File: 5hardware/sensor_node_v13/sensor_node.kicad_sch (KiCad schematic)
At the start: 42 parts, among them J1 Conn_01x08_Socket, J2 Conn_01x08_Socket, Q1 AO3400A, Q2 AO3401A, Q4 AO3401A, SW1 SW_Push, SW2 SW_Push, SW3 SW_Push, SW4 SW_Reed, SW5 SW_Push, SW6 SW_Push, SW7 SW_Push, U1 ESP-12F, U12 APDS-9960, U13 SHT31-DIS, U17 BH1750FVI-TR, U2 2N7002DW, U3 INA219AxDCN, U7 XC6206PxxxMR, U8 TPL5110

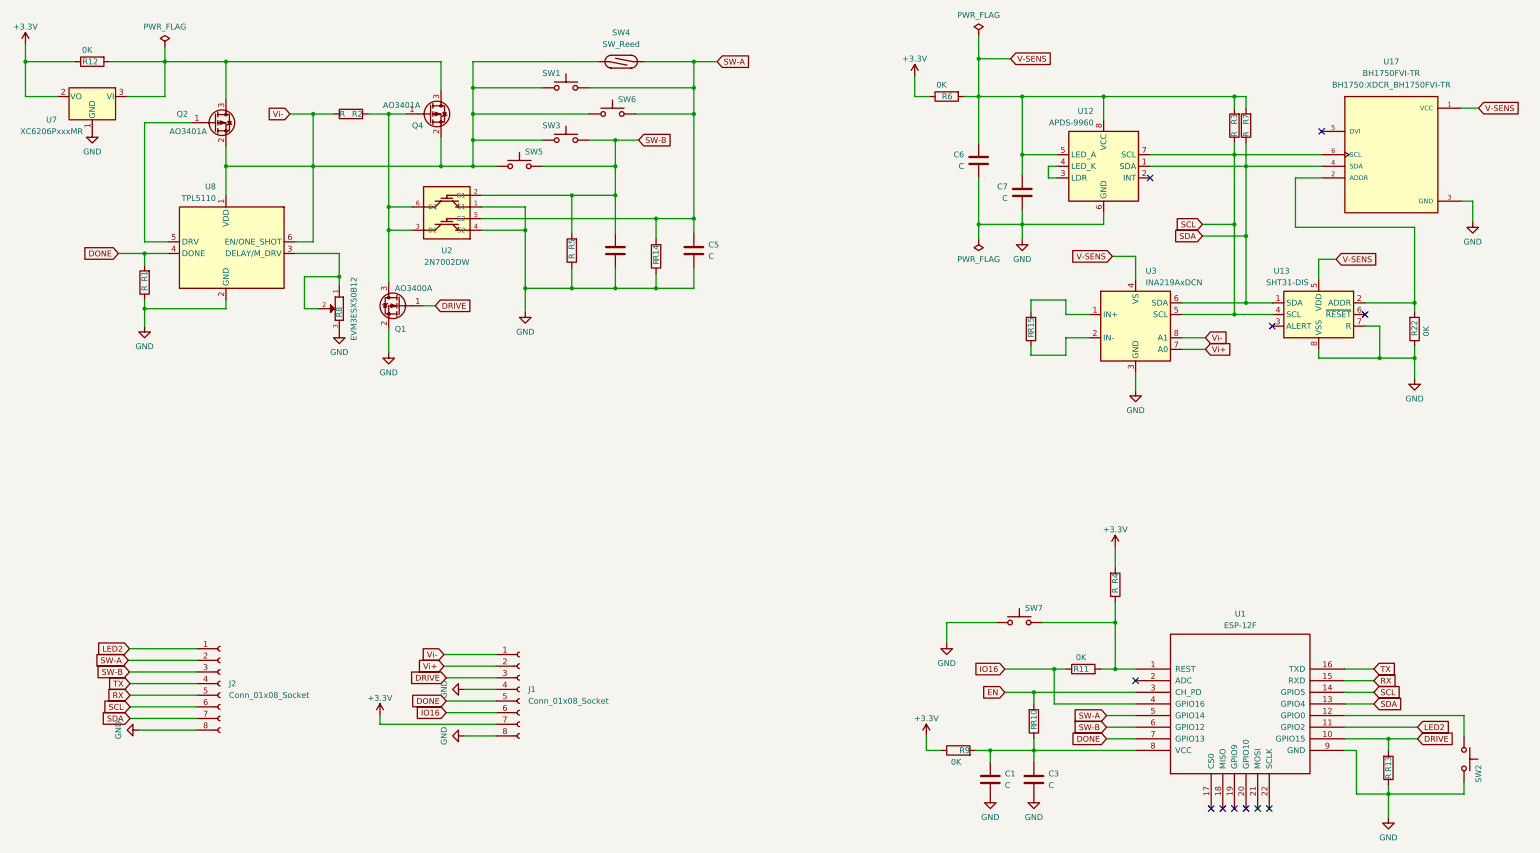
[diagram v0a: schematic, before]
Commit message: updated PCB.
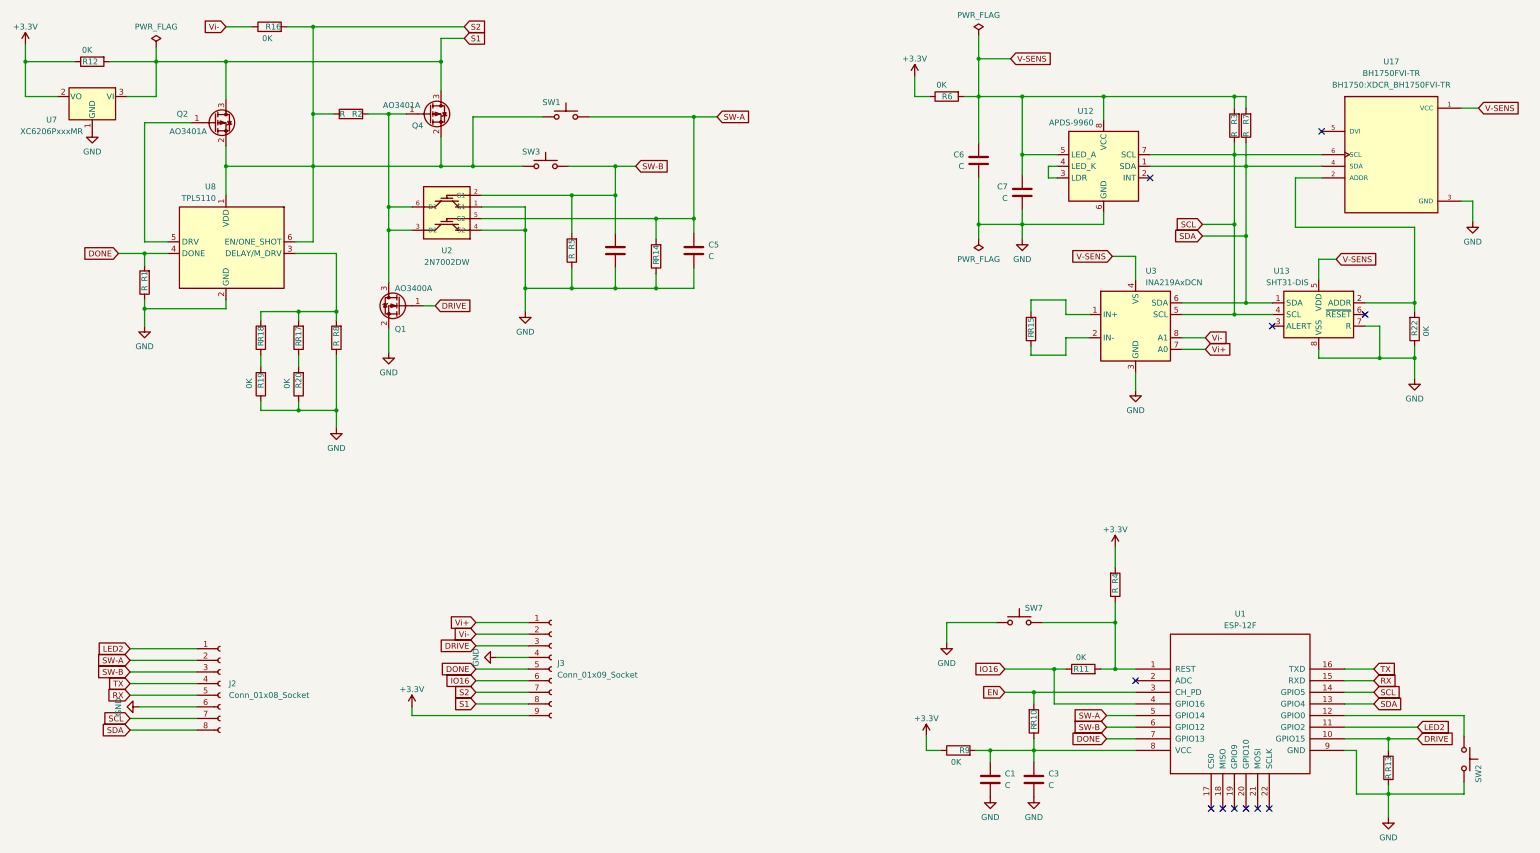
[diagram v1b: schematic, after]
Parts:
- removed J1: Conn_01x08_Socket, Connector_PinSocket_2.54mm:PinSocket_1x08_P2.54mm_Vertical, symbol Connector:Conn_01x08_Socket
- removed R8: EVM3ESX50B12, EVM3ES:EMV3ESX50B12, symbol EVM3ESX50B:EVM3ESX50B12
- removed SW4: SW_Reed, Button_Switch_SMD:SW_SPST_REED_CT10-XXXX-G1, symbol Switch:SW_Reed
- removed SW5, SW6: SW_Push, Button_Switch_SMD:SW_SPST_PTS810, symbol Switch:SW_Push
- added J3: Conn_01x09_Socket, Connector_PinSocket_2.54mm:PinSocket_1x09_P2.54mm_Vertical, symbol Connector:Conn_01x09_Socket
- added R16, R19, R20: 0K, Resistor_SMD:R_0402_1005Metric, symbol Device:R
- added R17, R18, R8: R, Resistor_SMD:R_0603_1608Metric, symbol Device:R
- R11, R12, R6, R9: footprint Resistor_SMD:R_0603_1608Metric -> Resistor_SMD:R_0402_1005Metric
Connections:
- net +3.3V: now also J3.9 (Pin_9)
- net DONE: now also J3.5 (Pin_5)
- net DRIVE: now also J3.3 (Pin_3)
- net GND: now also J2.6 (Pin_6), J3.4 (Pin_4), R19.1, R20.1, R8.1; no longer J2.8 (Pin_8)
- net IO16: now also J3.6 (Pin_6)
- net SCL: now also J2.7 (Pin_7); no longer J2.6 (Pin_6)
- net SDA: now also J2.8 (Pin_8); no longer J2.7 (Pin_7)
- net Vi+: now also J3.1 (Pin_1)
- net Vi-: now also J3.2 (Pin_2), R16.1; no longer Q2.2 (S), Q4.2 (S), R2.1, SW1.1, SW3.1, U8.1 (VDD), U8.6 (EN/ONE_SHOT)
- net at U8.3 (DELAY/M_DRV): now also R17.2, R18.2, R8.2
- net S1: now reaches Q2.3 (D), Q4.3 (D), R12.2, U7.3 (VI)
- net S1: now also J3.8 (Pin_8)
- new net: R18.1, R19.2
- new net: R17.1, R20.2
- new net S2: J3.7 (Pin_7), Q2.2 (S), Q4.2 (S), R16.2, R2.1, SW1.1, SW3.1, U8.1 (VDD), U8.6 (EN/ONE_SHOT)
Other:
- moved on the sheet: SW1, SW3
